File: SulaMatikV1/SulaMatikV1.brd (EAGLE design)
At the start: 66 x 61 mm, 43 parts, among them IC1 REG1117, Q1 2N3904, Q2 2N5551, Q3 2N5551

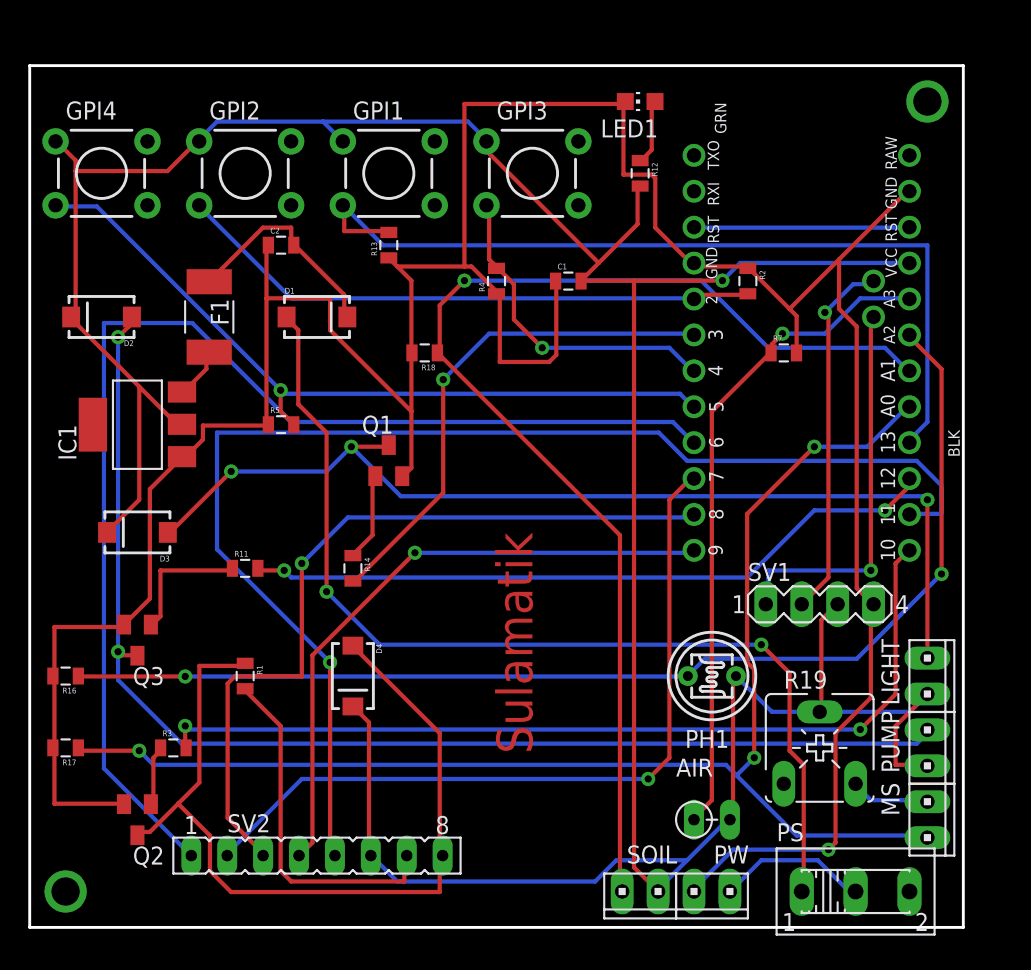
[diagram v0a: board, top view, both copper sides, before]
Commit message: v1
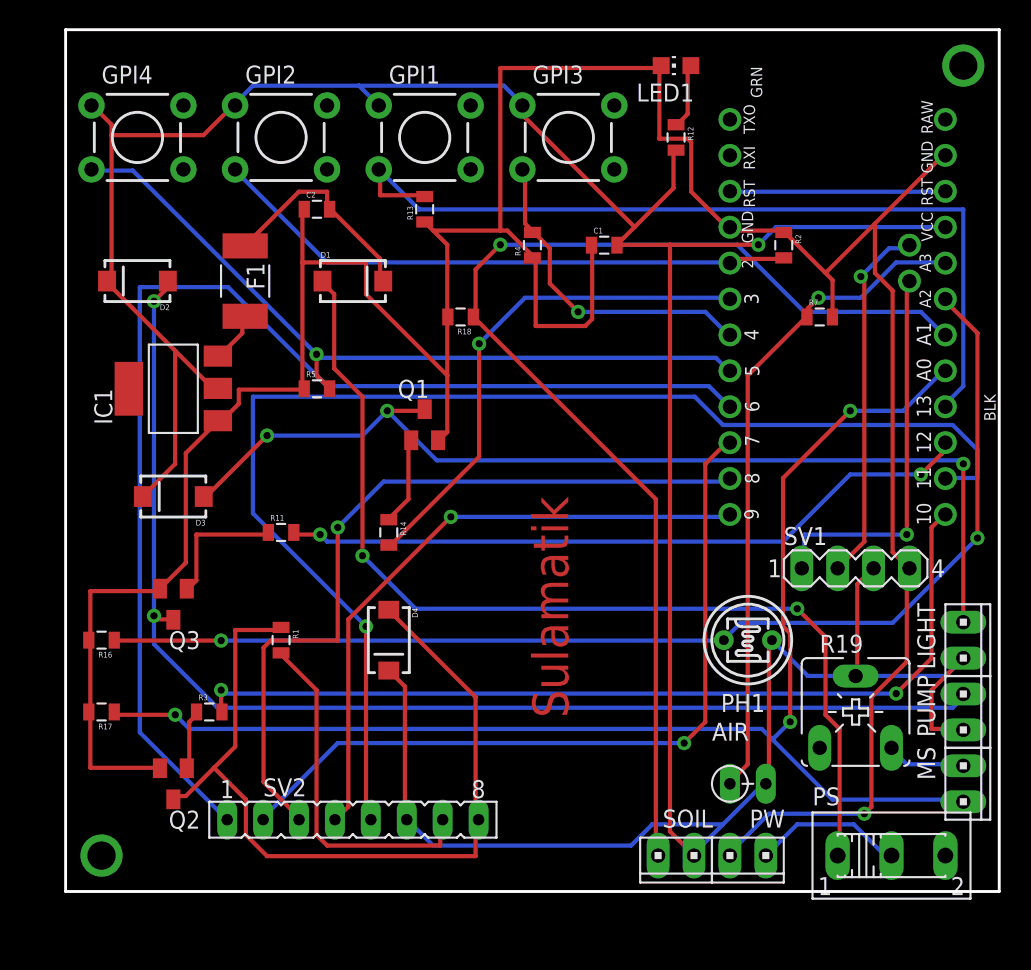
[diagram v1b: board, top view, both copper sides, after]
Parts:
- moved PUMP 3.59 mm to (66.0, 15.2)
- moved MS 3.59 mm to (66.0, 10.2)
- moved LIGHT 3.59 mm to (66.0, 20.3)
- moved R2 3.59 mm to (53.3, 48.3)
- moved R11 3.59 mm to (17.8, 27.9)
- moved GPI1 3.59 mm to (27.9, 55.9)
- moved Q1 3.59 mm to (27.9, 35.6)
- moved R13 3.59 mm to (27.9, 50.8)
- moved R14 3.59 mm to (25.4, 27.9)
- moved R17 3.59 mm to (5.08, 15.2)
- moved Q2 3.59 mm to (10.2, 10.2)
- moved AIR 3.59 mm to (50.8, 10.2)
- moved D2 3.59 mm to (7.62, 45.7)
- moved D3 3.59 mm to (10.2, 30.5)
- moved F1 3.59 mm to (15.2, 45.7)
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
